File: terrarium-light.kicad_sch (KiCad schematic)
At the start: 58 parts, among them J1 Conn_01x04_Pin, J2 USB_C_Receptacle_USB2.0_16P, Q1 UMH3N, SW1 RotaryEncoder_Switch_MP, U1 CH340C, U2 TPS61169DCKR, U3 TPS61169DCKR, U4 LM1117S-3.3, U6 ESP32-S3-MINI-1

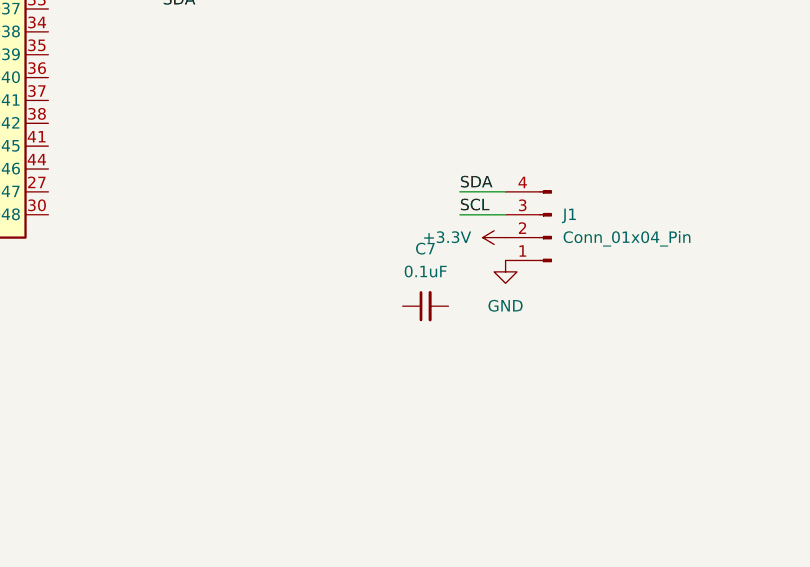
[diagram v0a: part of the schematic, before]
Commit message: saving
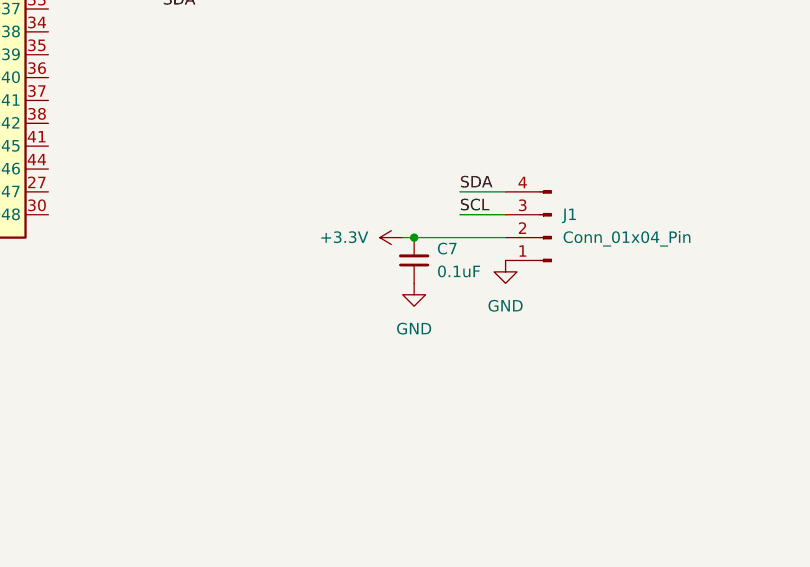
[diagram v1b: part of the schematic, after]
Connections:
- net +3.3V: now also C7.2
- net GND: now also C7.1
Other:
- moved on the sheet: C7
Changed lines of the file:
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@@
 	)
 	(junction
+		(at 111.76 107.95)
+		(diameter 0)
+		(color 0 0 0 0)
+	)
+	(junction
 		(at 271.78 114.3)
 		(diameter 0)
@@
 	(wire
 		(pts
+			(xy 111.76 107.95) (xy 121.92 107.95)
+		)
+		(stroke
+			(width 0)
+			(type default)
+		)
+	)
+	(wire
+		(pts
 			(xy 215.9 114.3) (xy 228.6 114.3)
 		)
@@
 	(wire
 		(pts
+			(xy 110.49 107.95) (xy 111.76 107.95)
+		)
+		(stroke
+			(width 0)
+			(type default)
+		)
+	)
+	(wire
+		(pts
 			(xy 215.9 50.8) (xy 228.6 50.8)
 		)
@@
 	(symbol
 		(lib_id "Device:C_Small")
-		(at 113.03 115.57 90)
+		(at 111.76 110.49 180)
 		(unit 1)
 		(exclude_from_sim no)
@@
 		(fields_autoplaced yes)
 		(property "Reference" "C7"
-			(at 113.0363 109.22 90)
+			(at 114.3 109.2135 0)
 			(effects
 				(font
 					(size 1.27 1.27)
 				)
+				(justify right)
 			)
 		)
 		(property "Value" "0.1uF "
-			(at 113.0363 111.76 90)
+			(at 114.3 111.7535 0)
 			(effects
 				(font
 					(size 1.27 1.27)
 				)
+				(justify right)
 			)
 		)
 		(property "Footprint" "Capacitor_SMD:C_0805_2012Metric_Pad1.18x1.45mm_HandSolder"
-			(at 113.03 115.57 0)
+			(at 111.76 110.49 0)
 			(effects
 				(font
@@
 		)
 		(property "Datasheet" "~"
-			(at 113.03 115.57 0)
+			(at 111.76 110.49 0)
 			(effects
 				(font
@@
 		)
 		(property "Description" "Unpolarized capacitor, small symbol"
-			(at 113.03 115.57 0)
+			(at 111.76 110.49 0)
 			(effects
 				(font
@@
 	(symbol
 		(lib_id "power:+3.3V")
-		(at 121.92 107.95 90)
+		(at 110.49 107.95 90)
 		(unit 1)
 		(exclude_from_sim no)
@@
 		(fields_autoplaced yes)
 		(property "Reference" "#PWR029"
-			(at 125.73 107.95 0)
+			(at 114.3 107.95 0)
 			(effects
 				(font
@@
 		)
 		(property "Value" "+3.3V"
-			(at 118.11 107.9499 90)
+			(at 106.68 107.9499 90)
 			(effects
 				(font
@@
 		)
 		(property "Footprint" ""
-			(at 121.92 107.95 0)
+			(at 110.49 107.95 0)
 			(effects
 				(font
@@
 		)
 		(property "Datasheet" ""
-			(at 121.92 107.95 0)
+			(at 110.49 107.95 0)
 			(effects
 				(font
@@
 		)
 		(property "Description" "Power symbol creates a global label with name \"+3.3V\""
-			(at 121.92 107.95 0)
+			(at 110.49 107.95 0)
 			(effects
 				(font
@@
 					(unit 1)
 				)
+			)
+		)
+	)
+	(symbol
+		(lib_id "power:GND")
+		(at 111.76 113.03 0)
+		(unit 1)
+		(exclude_from_sim no)
+		(in_bom yes)
+		(on_board yes)
+		(dnp no)
+		(fields_autoplaced yes)
+		(property "Reference" "#PWR036"
+			(at 111.76 119.38 0)
+			(effects
+				(font
+					(size 1.27 1.27)
+				)
+				(hide yes)
+			)
+		)
+		(property "Value" "GND"
+			(at 111.76 118.11 0)
+			(effects
+				(font
+					(size 1.27 1.27)
+				)
+			)
+		)
+		(property "Footprint" ""
+			(at 111.76 113.03 0)
+			(effects
+				(font
+					(size 1.27 1.27)
+				)
+				(hide yes)
+			)
+		)
+		(property "Datasheet" ""
+			(at 111.76 113.03 0)
+			(effects
+				(font
+					(size 1.27 1.27)
+				)
+				(hide yes)
+			)
+		)
+		(property "Description" "Power symbol creates a global label with name \"GND\" , ground"
+			(at 111.76 113.03 0)
+			(effects
+				(font
+					(size 1.27 1.27)
+				)
+				(hide yes)
+			)
+		)
+		(pin "1"
+		)
+		(instances
+			(project "terrarium-light"
+				(path "/15920752-a750-4c65-817e-4525ac22cfdb"
+					(reference "#PWR036")
+					(unit 1)
+				)
